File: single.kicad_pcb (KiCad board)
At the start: 2 copper layers, 17 x 14 mm, 8 parts, among them J1 Conn_01x01, J2 Conn_01x01, J3 Conn_01x01, J4 Conn_01x01, J5 Conn_01x01, J6 Conn_01x01

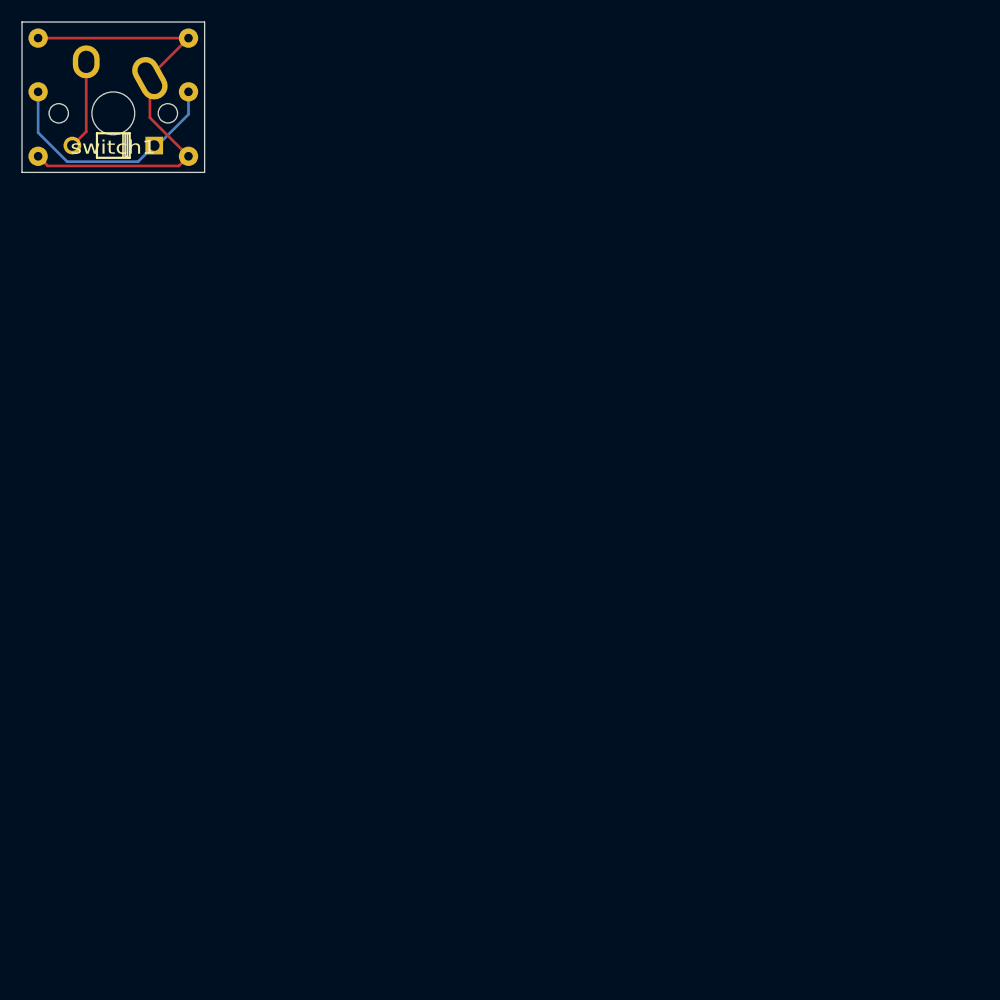
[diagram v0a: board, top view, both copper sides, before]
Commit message: 6x5.
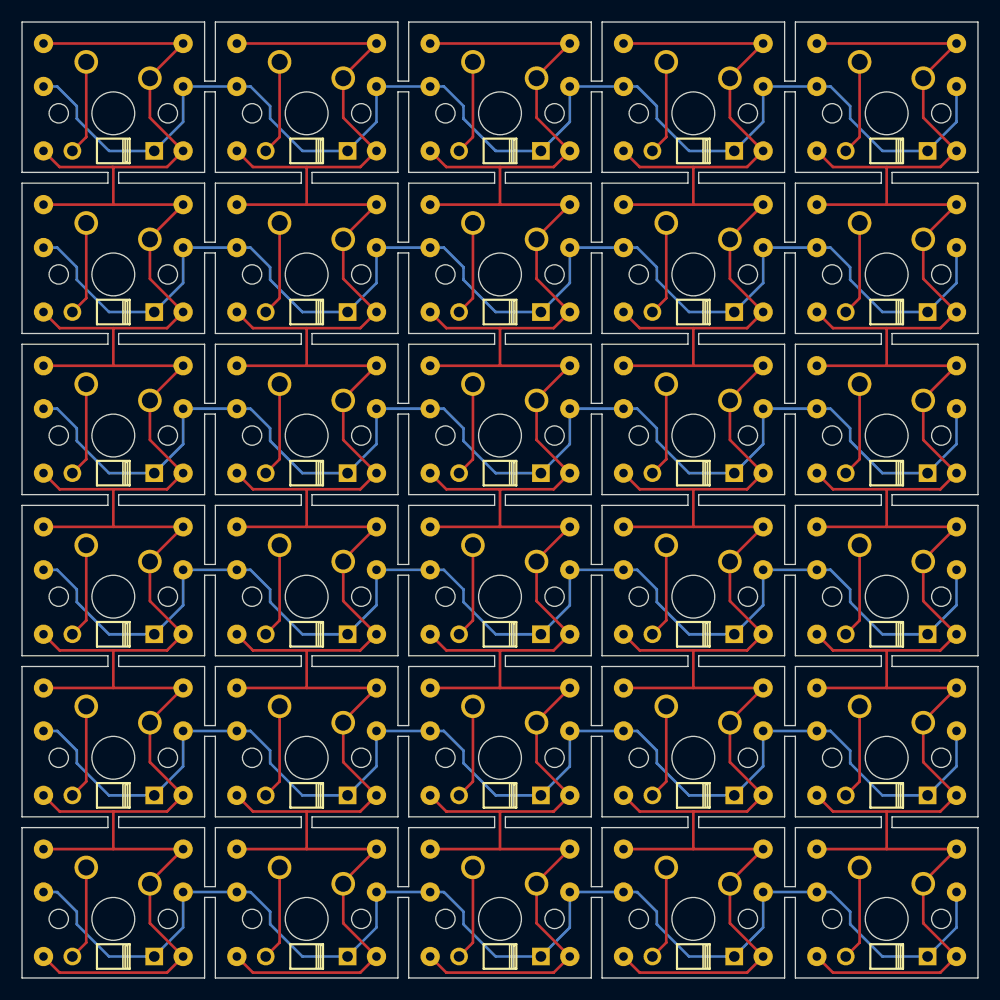
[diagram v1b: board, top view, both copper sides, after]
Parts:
- added J10: Conn_01x01, footprints:wirepad, F.Cu at (33.5, 103.5)
- added J100: Conn_01x01, footprints:wirepad, F.Cu at (105.5, 58.5)
- added J101: Conn_01x01, footprints:wirepad, F.Cu at (105.5, 63.5)
- added J102: Conn_01x01, footprints:wirepad, F.Cu at (105.5, 73.5)
- added J103: Conn_01x01, footprints:wirepad, F.Cu at (105.5, 78.5)
- added J104: Conn_01x01, footprints:wirepad, F.Cu at (105.5, 88.5)
- added J105: Conn_01x01, footprints:wirepad, F.Cu at (105.5, 93.5)
- added J106: Conn_01x01, footprints:wirepad, F.Cu at (105.5, 103.5)
- added J107: Conn_01x01, footprints:wirepad, F.Cu at (105.5, 108.5)
- added J108: Conn_01x01, footprints:wirepad, F.Cu at (105.5, 118.5)
- added J109: Conn_01x01, footprints:wirepad, F.Cu at (118.5, 33.5)
- added J11: Conn_01x01, footprints:wirepad, F.Cu at (33.5, 108.5)
- added J110: Conn_01x01, footprints:wirepad, F.Cu at (118.5, 43.5)
- added J111: Conn_01x01, footprints:wirepad, F.Cu at (118.5, 48.5)
- added J112: Conn_01x01, footprints:wirepad, F.Cu at (118.5, 58.5)
- added J113: Conn_01x01, footprints:wirepad, F.Cu at (118.5, 63.5)
- added J114: Conn_01x01, footprints:wirepad, F.Cu at (118.5, 73.5)
- added J115: Conn_01x01, footprints:wirepad, F.Cu at (118.5, 78.5)
- added J116: Conn_01x01, footprints:wirepad, F.Cu at (118.5, 88.5)
- added J117: Conn_01x01, footprints:wirepad, F.Cu at (118.5, 93.5)
- added J118: Conn_01x01, footprints:wirepad, F.Cu at (118.5, 103.5)
- added J119: Conn_01x01, footprints:wirepad, F.Cu at (118.5, 108.5)
- added J12: Conn_01x01, footprints:wirepad, F.Cu at (33.5, 118.5)
- added J120: Conn_01x01, footprints:wirepad, F.Cu at (118.5, 118.5)
- added J121: Conn_01x01, footprints:wirepad, F.Cu at (33.5, 37.5)
- added J122: Conn_01x01, footprints:wirepad, F.Cu at (46.5, 37.5)
- added J123: Conn_01x01, footprints:wirepad, F.Cu at (33.5, 52.5)
- added J124: Conn_01x01, footprints:wirepad, F.Cu at (46.5, 52.5)
- added J125: Conn_01x01, footprints:wirepad, F.Cu at (33.5, 67.5)
- added J126: Conn_01x01, footprints:wirepad, F.Cu at (46.5, 67.5)
- added J127: Conn_01x01, footprints:wirepad, F.Cu at (33.5, 82.5)
- added J128: Conn_01x01, footprints:wirepad, F.Cu at (46.5, 82.5)
- added J129: Conn_01x01, footprints:wirepad, F.Cu at (33.5, 97.5)
- added J13: Conn_01x01, footprints:wirepad, F.Cu at (46.5, 33.5)
- added J130: Conn_01x01, footprints:wirepad, F.Cu at (46.5, 97.5)
- added J131: Conn_01x01, footprints:wirepad, F.Cu at (51.5, 37.5)
- added J132: Conn_01x01, footprints:wirepad, F.Cu at (64.5, 37.5)
- added J133: Conn_01x01, footprints:wirepad, F.Cu at (51.5, 52.5)
- added J134: Conn_01x01, footprints:wirepad, F.Cu at (64.5, 52.5)
- added J135: Conn_01x01, footprints:wirepad, F.Cu at (51.5, 67.5)
- added J136: Conn_01x01, footprints:wirepad, F.Cu at (64.5, 67.5)
- added J137: Conn_01x01, footprints:wirepad, F.Cu at (51.5, 82.5)
- added J138: Conn_01x01, footprints:wirepad, F.Cu at (64.5, 82.5)
- added J139: Conn_01x01, footprints:wirepad, F.Cu at (51.5, 97.5)
- added J14: Conn_01x01, footprints:wirepad, F.Cu at (46.5, 43.5)
- added J140: Conn_01x01, footprints:wirepad, F.Cu at (64.5, 97.5)
- added J141: Conn_01x01, footprints:wirepad, F.Cu at (69.5, 37.5)
- added J142: Conn_01x01, footprints:wirepad, F.Cu at (82.5, 37.5)
- added J143: Conn_01x01, footprints:wirepad, F.Cu at (69.5, 52.5)
- added J144: Conn_01x01, footprints:wirepad, F.Cu at (82.5, 52.5)
- added J145: Conn_01x01, footprints:wirepad, F.Cu at (69.5, 67.5)
- added J146: Conn_01x01, footprints:wirepad, F.Cu at (82.5, 67.5)
- added J147: Conn_01x01, footprints:wirepad, F.Cu at (69.5, 82.5)
- added J148: Conn_01x01, footprints:wirepad, F.Cu at (82.5, 82.5)
- added J149: Conn_01x01, footprints:wirepad, F.Cu at (69.5, 97.5)
- added J15: Conn_01x01, footprints:wirepad, F.Cu at (46.5, 48.5)
- added J150: Conn_01x01, footprints:wirepad, F.Cu at (82.5, 97.5)
- added J151: Conn_01x01, footprints:wirepad, F.Cu at (87.5, 37.5)
- added J152: Conn_01x01, footprints:wirepad, F.Cu at (100.5, 37.5)
- added J153: Conn_01x01, footprints:wirepad, F.Cu at (87.5, 52.5)
- added J154: Conn_01x01, footprints:wirepad, F.Cu at (100.5, 52.5)
- added J155: Conn_01x01, footprints:wirepad, F.Cu at (87.5, 67.5)
- added J156: Conn_01x01, footprints:wirepad, F.Cu at (100.5, 67.5)
- added J157: Conn_01x01, footprints:wirepad, F.Cu at (87.5, 82.5)
- added J158: Conn_01x01, footprints:wirepad, F.Cu at (100.5, 82.5)
- added J159: Conn_01x01, footprints:wirepad, F.Cu at (87.5, 97.5)
- added J16: Conn_01x01, footprints:wirepad, F.Cu at (46.5, 58.5)
- added J160: Conn_01x01, footprints:wirepad, F.Cu at (105.5, 97.5)
- added J161: Conn_01x01, footprints:wirepad, F.Cu at (105.5, 37.5)
- added J162: Conn_01x01, footprints:wirepad, F.Cu at (118.5, 37.5)
- added J163: Conn_01x01, footprints:wirepad, F.Cu at (105.5, 52.5)
- added J164: Conn_01x01, footprints:wirepad, F.Cu at (118.5, 52.5)
- added J165: Conn_01x01, footprints:wirepad, F.Cu at (105.5, 67.5)
- added J166: Conn_01x01, footprints:wirepad, F.Cu at (118.5, 67.5)
- added J167: Conn_01x01, footprints:wirepad, F.Cu at (105.5, 82.5)
- added J168: Conn_01x01, footprints:wirepad, F.Cu at (118.5, 82.5)
- added J169: Conn_01x01, footprints:wirepad, F.Cu at (100.5, 97.5)
- added J17: Conn_01x01, footprints:wirepad, F.Cu at (46.5, 63.5)
- added J170: Conn_01x01, footprints:wirepad, F.Cu at (118.5, 97.5)
- added J171: Conn_01x01, footprints:wirepad, F.Cu at (33.5, 112.5)
- added J172: Conn_01x01, footprints:wirepad, F.Cu at (46.5, 112.5)
- added J173: Conn_01x01, footprints:wirepad, F.Cu at (51.5, 112.5)
- added J174: Conn_01x01, footprints:wirepad, F.Cu at (64.5, 112.5)
- added J175: Conn_01x01, footprints:wirepad, F.Cu at (69.5, 112.5)
- added J176: Conn_01x01, footprints:wirepad, F.Cu at (82.5, 112.5)
- added J177: Conn_01x01, footprints:wirepad, F.Cu at (87.5, 112.5)
- added J178: Conn_01x01, footprints:wirepad, F.Cu at (100.5, 112.5)
- added J179: Conn_01x01, footprints:wirepad, F.Cu at (105.5, 112.5)
- added J18: Conn_01x01, footprints:wirepad, F.Cu at (46.5, 73.5)
- added J180: Conn_01x01, footprints:wirepad, F.Cu at (118.5, 112.5)
- added J19: Conn_01x01, footprints:wirepad, F.Cu at (46.5, 78.5)
- added J20: Conn_01x01, footprints:wirepad, F.Cu at (46.5, 88.5)
- added J21: Conn_01x01, footprints:wirepad, F.Cu at (46.5, 93.5)
- added J22: Conn_01x01, footprints:wirepad, F.Cu at (46.5, 103.5)
- added J23: Conn_01x01, footprints:wirepad, F.Cu at (46.5, 108.5)
- added J24: Conn_01x01, footprints:wirepad, F.Cu at (46.5, 118.5)
- added J25: Conn_01x01, footprints:wirepad, F.Cu at (51.5, 33.5)
- added J26: Conn_01x01, footprints:wirepad, F.Cu at (51.5, 43.5)
- added J27: Conn_01x01, footprints:wirepad, F.Cu at (51.5, 48.5)
- added J28: Conn_01x01, footprints:wirepad, F.Cu at (51.5, 58.5)
- added J29: Conn_01x01, footprints:wirepad, F.Cu at (51.5, 63.5)
- added J30: Conn_01x01, footprints:wirepad, F.Cu at (51.5, 73.5)
- added J31: Conn_01x01, footprints:wirepad, F.Cu at (51.5, 78.5)
- added J32: Conn_01x01, footprints:wirepad, F.Cu at (51.5, 88.5)
- added J33: Conn_01x01, footprints:wirepad, F.Cu at (51.5, 93.5)
- added J34: Conn_01x01, footprints:wirepad, F.Cu at (51.5, 103.5)
- added J35: Conn_01x01, footprints:wirepad, F.Cu at (51.5, 108.5)
- added J36: Conn_01x01, footprints:wirepad, F.Cu at (51.5, 118.5)
- added J37: Conn_01x01, footprints:wirepad, F.Cu at (64.5, 33.5)
- added J38: Conn_01x01, footprints:wirepad, F.Cu at (64.5, 43.5)
- added J39: Conn_01x01, footprints:wirepad, F.Cu at (64.5, 48.5)
- added J40: Conn_01x01, footprints:wirepad, F.Cu at (64.5, 58.5)
- added J41: Conn_01x01, footprints:wirepad, F.Cu at (64.5, 63.5)
- added J42: Conn_01x01, footprints:wirepad, F.Cu at (64.5, 73.5)
- added J43: Conn_01x01, footprints:wirepad, F.Cu at (64.5, 78.5)
- added J44: Conn_01x01, footprints:wirepad, F.Cu at (64.5, 88.5)
- added J45: Conn_01x01, footprints:wirepad, F.Cu at (64.5, 93.5)
- added J46: Conn_01x01, footprints:wirepad, F.Cu at (64.5, 103.5)
- added J47: Conn_01x01, footprints:wirepad, F.Cu at (64.5, 108.5)
- added J48: Conn_01x01, footprints:wirepad, F.Cu at (64.5, 118.5)
- added J49: Conn_01x01, footprints:wirepad, F.Cu at (69.5, 33.5)
- added J50: Conn_01x01, footprints:wirepad, F.Cu at (69.5, 43.5)
- added J51: Conn_01x01, footprints:wirepad, F.Cu at (69.5, 48.5)
- added J52: Conn_01x01, footprints:wirepad, F.Cu at (69.5, 58.5)
- added J53: Conn_01x01, footprints:wirepad, F.Cu at (69.5, 63.5)
- added J54: Conn_01x01, footprints:wirepad, F.Cu at (69.5, 73.5)
- added J55: Conn_01x01, footprints:wirepad, F.Cu at (69.5, 78.5)
- added J56: Conn_01x01, footprints:wirepad, F.Cu at (69.5, 88.5)
- added J57: Conn_01x01, footprints:wirepad, F.Cu at (69.5, 93.5)
- added J58: Conn_01x01, footprints:wirepad, F.Cu at (69.5, 103.5)
- added J59: Conn_01x01, footprints:wirepad, F.Cu at (69.5, 108.5)
- added J60: Conn_01x01, footprints:wirepad, F.Cu at (69.5, 118.5)
- added J61: Conn_01x01, footprints:wirepad, F.Cu at (82.5, 33.5)
- added J62: Conn_01x01, footprints:wirepad, F.Cu at (82.5, 43.5)
- added J63: Conn_01x01, footprints:wirepad, F.Cu at (82.5, 48.5)
- added J64: Conn_01x01, footprints:wirepad, F.Cu at (82.5, 58.5)
- added J65: Conn_01x01, footprints:wirepad, F.Cu at (82.5, 63.5)
- added J66: Conn_01x01, footprints:wirepad, F.Cu at (82.5, 73.5)
- added J67: Conn_01x01, footprints:wirepad, F.Cu at (82.5, 78.5)
- added J68: Conn_01x01, footprints:wirepad, F.Cu at (82.5, 88.5)
- added J69: Conn_01x01, footprints:wirepad, F.Cu at (82.5, 93.5)
- added J7: Conn_01x01, footprints:wirepad, F.Cu at (33.5, 78.5)
- added J70: Conn_01x01, footprints:wirepad, F.Cu at (82.5, 103.5)
- added J71: Conn_01x01, footprints:wirepad, F.Cu at (82.5, 108.5)
- added J72: Conn_01x01, footprints:wirepad, F.Cu at (82.5, 118.5)
- added J73: Conn_01x01, footprints:wirepad, F.Cu at (87.5, 33.5)
- added J74: Conn_01x01, footprints:wirepad, F.Cu at (87.5, 43.5)
- added J75: Conn_01x01, footprints:wirepad, F.Cu at (87.5, 48.5)
- added J76: Conn_01x01, footprints:wirepad, F.Cu at (87.5, 58.5)
- added J77: Conn_01x01, footprints:wirepad, F.Cu at (87.5, 63.5)
- added J78: Conn_01x01, footprints:wirepad, F.Cu at (87.5, 73.5)
- added J79: Conn_01x01, footprints:wirepad, F.Cu at (87.5, 78.5)
- added J8: Conn_01x01, footprints:wirepad, F.Cu at (33.5, 88.5)
- added J80: Conn_01x01, footprints:wirepad, F.Cu at (87.5, 88.5)
- added J81: Conn_01x01, footprints:wirepad, F.Cu at (87.5, 93.5)
- added J82: Conn_01x01, footprints:wirepad, F.Cu at (87.5, 103.5)
- added J83: Conn_01x01, footprints:wirepad, F.Cu at (87.5, 108.5)
- added J84: Conn_01x01, footprints:wirepad, F.Cu at (87.5, 118.5)
- added J85: Conn_01x01, footprints:wirepad, F.Cu at (100.5, 33.5)
- added J86: Conn_01x01, footprints:wirepad, F.Cu at (100.5, 43.5)
- added J87: Conn_01x01, footprints:wirepad, F.Cu at (100.5, 48.5)
- added J88: Conn_01x01, footprints:wirepad, F.Cu at (100.5, 58.5)
- added J89: Conn_01x01, footprints:wirepad, F.Cu at (100.5, 63.5)
- added J9: Conn_01x01, footprints:wirepad, F.Cu at (33.5, 93.5)
- added J90: Conn_01x01, footprints:wirepad, F.Cu at (100.5, 73.5)
- added J91: Conn_01x01, footprints:wirepad, F.Cu at (100.5, 78.5)
- added J92: Conn_01x01, footprints:wirepad, F.Cu at (100.5, 88.5)
- added J93: Conn_01x01, footprints:wirepad, F.Cu at (100.5, 93.5)
- added J94: Conn_01x01, footprints:wirepad, F.Cu at (100.5, 103.5)
- added J95: Conn_01x01, footprints:wirepad, F.Cu at (100.5, 108.5)
- added J96: Conn_01x01, footprints:wirepad, F.Cu at (100.5, 118.5)
- added J97: Conn_01x01, footprints:wirepad, F.Cu at (105.5, 33.5)
- added J98: Conn_01x01, footprints:wirepad, F.Cu at (105.5, 43.5)
- added J99: Conn_01x01, footprints:wirepad, F.Cu at (105.5, 48.5)
- added diode10: diode, footprints:diode, F.Cu at (58.0, 88.5)
- added diode11: diode, footprints:diode, F.Cu at (58.0, 103.5)
- added diode12: diode, footprints:diode, F.Cu at (58.0, 118.5)
- added diode13: diode, footprints:diode, F.Cu at (76.0, 43.5)
- added diode14: diode, footprints:diode, F.Cu at (76.0, 58.5)
- added diode15: diode, footprints:diode, F.Cu at (76.0, 73.5)
- added diode16: diode, footprints:diode, F.Cu at (76.0, 88.5)
- added diode17: diode, footprints:diode, F.Cu at (76.0, 103.5)
- added diode18: diode, footprints:diode, F.Cu at (76.0, 118.5)
- added diode19: diode, footprints:diode, F.Cu at (94.0, 43.5)
- added diode2: diode, footprints:diode, F.Cu at (40.0, 58.5)
- added diode20: diode, footprints:diode, F.Cu at (94.0, 58.5)
- added diode21: diode, footprints:diode, F.Cu at (94.0, 73.5)
- added diode22: diode, footprints:diode, F.Cu at (94.0, 88.5)
- added diode23: diode, footprints:diode, F.Cu at (94.0, 103.5)
- added diode24: diode, footprints:diode, F.Cu at (94.0, 118.5)
- added diode25: diode, footprints:diode, F.Cu at (112.0, 43.5)
- added diode26: diode, footprints:diode, F.Cu at (112.0, 58.5)
- added diode27: diode, footprints:diode, F.Cu at (112.0, 73.5)
- added diode28: diode, footprints:diode, F.Cu at (112.0, 88.5)
- added diode29: diode, footprints:diode, F.Cu at (112.0, 103.5)
- added diode3: diode, footprints:diode, F.Cu at (40.0, 73.5)
- added diode30: diode, footprints:diode, F.Cu at (112.0, 118.5)
- added diode4: diode, footprints:diode, F.Cu at (40.0, 88.5)
- added diode5: diode, footprints:diode, F.Cu at (40.0, 103.5)
- added diode6: diode, footprints:diode, F.Cu at (40.0, 118.5)
- added diode7: diode, footprints:diode, F.Cu at (58.0, 43.5)
- added diode8: diode, footprints:diode, F.Cu at (58.0, 58.5)
- added diode9: diode, footprints:diode, F.Cu at (58.0, 73.5)
- added switch10: switch, footprints:1u-minimal, F.Cu at (58.0, 85.0)
- added switch11: switch, footprints:1u-minimal, F.Cu at (58.0, 100.0)
- added switch12: switch, footprints:1u-minimal, F.Cu at (58.0, 115.0)
- added switch13: switch, footprints:1u-minimal, F.Cu at (76.0, 40.0)
- added switch14: switch, footprints:1u-minimal, F.Cu at (76.0, 55.0)
- added switch15: switch, footprints:1u-minimal, F.Cu at (76.0, 70.0)
- added switch16: switch, footprints:1u-minimal, F.Cu at (76.0, 85.0)
- added switch17: switch, footprints:1u-minimal, F.Cu at (76.0, 100.0)
- added switch18: switch, footprints:1u-minimal, F.Cu at (76.0, 115.0)
- added switch19: switch, footprints:1u-minimal, F.Cu at (94.0, 40.0)
- added switch2: switch, footprints:1u-minimal, F.Cu at (40.0, 55.0)
- added switch20: switch, footprints:1u-minimal, F.Cu at (94.0, 55.0)
- added switch21: switch, footprints:1u-minimal, F.Cu at (94.0, 70.0)
- added switch22: switch, footprints:1u-minimal, F.Cu at (94.0, 85.0)
- added switch23: switch, footprints:1u-minimal, F.Cu at (94.0, 100.0)
- added switch24: switch, footprints:1u-minimal, F.Cu at (94.0, 115.0)
- added switch25: switch, footprints:1u-minimal, F.Cu at (112.0, 40.0)
- added switch26: switch, footprints:1u-minimal, F.Cu at (112.0, 55.0)
- added switch27: switch, footprints:1u-minimal, F.Cu at (112.0, 70.0)
- added switch28: switch, footprints:1u-minimal, F.Cu at (112.0, 85.0)
- added switch29: switch, footprints:1u-minimal, F.Cu at (112.0, 100.0)
- added switch3: switch, footprints:1u-minimal, F.Cu at (40.0, 70.0)
- added switch30: switch, footprints:1u-minimal, F.Cu at (112.0, 115.0)
- added switch4: switch, footprints:1u-minimal, F.Cu at (40.0, 85.0)
- added switch5: switch, footprints:1u-minimal, F.Cu at (40.0, 100.0)
- added switch6: switch, footprints:1u-minimal, F.Cu at (40.0, 115.0)
- added switch7: switch, footprints:1u-minimal, F.Cu at (58.0, 40.0)
- added switch8: switch, footprints:1u-minimal, F.Cu at (58.0, 55.0)
- added switch9: switch, footprints:1u-minimal, F.Cu at (58.0, 70.0)
- switch1: footprint footprints:1u-flipped -> footprints:1u-minimal
- moved J5 33.4 mm to (33.5, 63.5)
- moved J6 32.4 mm to (33.5, 73.5)
- moved J4 20.5 mm to (33.5, 58.5)
- moved J1 14.2 mm to (33.5, 33.5)
- moved J2 10.5 mm to (33.5, 43.5)
- moved J3 4.53 mm to (33.5, 48.5)
- moved diode1 0.50 mm to (40.0, 43.5)
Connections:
- J2 pad 1: Net-(J2-Pad1) -> Net-(J1-Pad1)
- J3 pad 1: Net-(J2-Pad1) -> Net-(J1-Pad1)
- J5 pad 1: Net-(J2-Pad1) -> Net-(J1-Pad1)
- J6 pad 1: Net-(J2-Pad1) -> Net-(J1-Pad1)
- diode1 pad 1: Net-(J1-Pad1) -> Net-(J121-Pad1)
- switch1 pad 2: Net-(J2-Pad1) -> Net-(J1-Pad1)
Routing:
- net Net-(J73-Pad1): track 0.00 -> 255.5 mm
- net Net-(J49-Pad1): track 0.00 -> 255.5 mm
- net Net-(J100-Pad1): track 0.00 -> 255.5 mm
- net Net-(J25-Pad1): track 0.00 -> 255.5 mm
- net Net-(J1-Pad1): track 22.8 -> 255.7 mm
- net Net-(J121-Pad1): track 0.00 -> 122.9 mm
- net Net-(J123-Pad1): track 0.00 -> 122.9 mm
- net Net-(J171-Pad1): track 0.00 -> 122.9 mm
- net Net-(J129-Pad1): track 0.00 -> 122.9 mm
- net Net-(J127-Pad1): track 0.00 -> 122.9 mm
- net Net-(J125-Pad1): track 0.00 -> 122.9 mm
- net Net-(J2-Pad1): track 42.7 -> 0.00 mm
- net Net-(diode30-Pad2): track 0.00 -> 8.82 mm
- net Net-(diode29-Pad2): track 0.00 -> 8.82 mm
- net Net-(diode28-Pad2): track 0.00 -> 8.82 mm
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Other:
- board size 17 x 14 mm -> 89 x 89 mm
